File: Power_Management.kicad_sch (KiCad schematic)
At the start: 30 parts, among them IC2 OpAmp_NE5532D, Q1 MOSFET_SI2333DDS-T1-BE3

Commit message: Update
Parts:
- removed C25, C27: 10u, Capacitor_SMD:C_0805_2012Metric, symbol Device:C
- removed C30: 470n, Capacitor_SMD:C_0805_2012Metric, symbol Device:C
- removed D1: SMAJ6.0A, Personal_Project:DO-214AC-2, symbol Personal_Projects:DIODE_SMAJ6.0A
- removed JST1: JST_S3B-XH-2.54, Personal_Project:JST_S3B-XH-SHDRRA3W64P0X250_1X3_990X1150X610P, symbol Personal_Projects:JST_S3B-XH-A-1_LF_SN
- removed LDO3: LDO_LD39200PU33R, Package_DFN_QFN:DFN-6-1EP_3x3mm_P0.95mm_EP1.7x2.6mm, symbol Personal_Projects:LDO_LD39200PU33R
- removed Q1: MOSFET_SI2333DDS-T1-BE3, Personal_Project:MOSFET_ SI2333DDS_SOT_DS-T1-BE3_VIS, symbol Personal_Projects:MOSFET_SI2333DDS-T1-BE3
- removed R12: 100k, Resistor_SMD:R_0805_2012Metric, symbol Device:R
- removed R13: 90k, Resistor_SMD:R_0805_2012Metric, symbol Device:R
- removed R14: 10k, Resistor_SMD:R_0805_2012Metric, symbol Device:R
- removed S2: Switch_WS-SLSU SMT Mini Slide, Personal_Project:Switch_WS-SLSU SMT Mini Slide, symbol Personal_Projects:Switch_WS-SLSU SMT Mini Slide
- removed Z1: Diode_BZX84C6V2-7-F, Personal_Project:Diode_BZX84C6V2_SOT96P240X110-3N, symbol Personal_Projects:Diode_BZX84C6V2-7-F
- added D2: SMAJ6.0A, Personal_Project:DO-214AC-2, symbol Personal_Projects:DIODE_SMAJ6.0A
- added JST2: JST_S3B-XH-2.54, Personal_Project:JST_S3B-XH-SHDRRA3W64P0X250_1X3_990X1150X610P, symbol Personal_Projects:JST_S3B-XH-A-1_LF_SN
- added Q2: MOSFET_SI2333DDS-T1-BE3, Personal_Project:MOSFET_ SI2333DDS_SOT_DS-T1-BE3_VIS, symbol Personal_Projects:MOSFET_SI2333DDS-T1-BE3
- added R7: 100k, Resistor_SMD:R_0805_2012Metric, symbol Device:R
- added U1: SN74LVC1G07DBVR, Package_TO_SOT_SMD:SOT-23-5, symbol 74xGxx:74LVC1G07
- added Z2: Diode_BZX84C6V2-7-F, Personal_Project:Diode_BZX84C6V2_SOT96P240X110-3N, symbol Personal_Projects:Diode_BZX84C6V2-7-F
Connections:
- net *RST: now also U1.4
- net +3.3V: now also U1.5 (VCC)
- net GND: now also D2.2 (A), JST2.2 (PWR-), R7.2, U1.3 (GND)
- net PWR+: now also JST2.1 (PWR+), Q2.3 (D)
- net VIN_LDLN050PUR renamed PWR+_PP
- net PWR+_PP: now also D2.1 (K), Q2.2 (S), Z2.3 (K)
- new net PWR+_GATE: Q2.1 (G), R7.1, Z2.1 (A)
- new net RST_PWR: JST2.3 (RST), U1.2
- no-connect marks 11 -> 7
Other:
- note added: "NO PU"
- note removed: "ON/OFF Switch"
- note removed: "Pin 2 connects to one or three"
- note removed: "VIN from 1.25 V to 6.0 V"
- moved on the sheet: C1, C17, C18, C21, IC2, LDO2, VS2

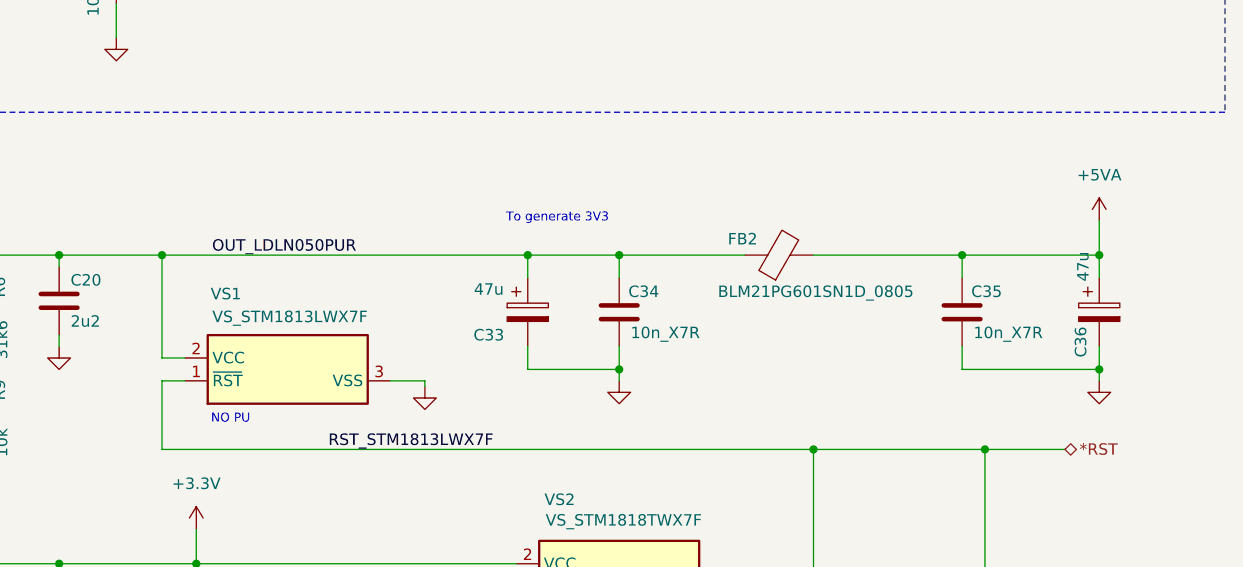
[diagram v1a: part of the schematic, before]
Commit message: Update
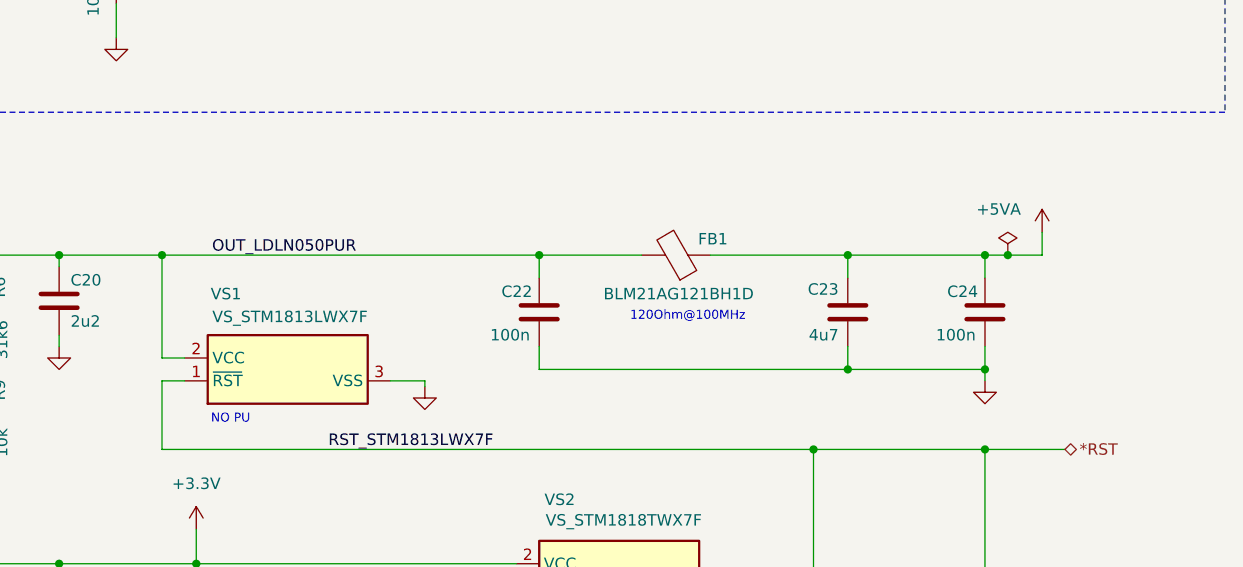
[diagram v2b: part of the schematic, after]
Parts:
- removed C33, C36: 47u, Capacitor_SMD:C_0805_2012Metric, symbol Device:C_Polarized
- removed C34, C35: 10n_X7R, Capacitor_SMD:C_0805_2012Metric, symbol Device:C
- removed FB2: BLM21PG601SN1D_0805, Capacitor_SMD:C_0805_2012Metric, symbol Device:FerriteBead
- added C22, C24: 100n, Capacitor_SMD:C_0805_2012Metric, symbol Device:C
- added C23: 4u7, Capacitor_SMD:C_0805_2012Metric, symbol Device:C
- added FB1: BLM21AG121BH1D, Capacitor_SMD:C_0805_2012Metric, symbol Device:FerriteBead
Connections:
- net +5VA: now also C23.1, C24.1, FB1.1
- net GND: now also C22.2, C23.2, C24.2
- net OUT_LDLN050PUR: now also C22.1, FB1.2
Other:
- note added: "120Ohm@100MHz"
- note removed: "To generate 3V3"
